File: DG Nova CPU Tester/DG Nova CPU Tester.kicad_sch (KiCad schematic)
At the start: 122 parts, among them J1 Slot_02x50_Odd_Even, J10 Programmed I/O, J11 CPU Option Inputs, J12 Data Channel, J13 Program Interrupt, J14 System Control, J17 CPU Option Outputs, J18 MEM Control Outputs, J19 Logic 8 CH, J20 Logic 8 CH, J21 Arduino Anolog Pins, J22 Arduino Digital Pins, J23 Arduino Digital Pins, J4 ATX Power Port, J6 MBO, J7 MEM, J8 Data Channel, J9 Front Panel Controls, SW1 Arduino Mega Reset, SW1 Pico Reset, SW2 Power Swtich, U1 74HC14, U2 Pico

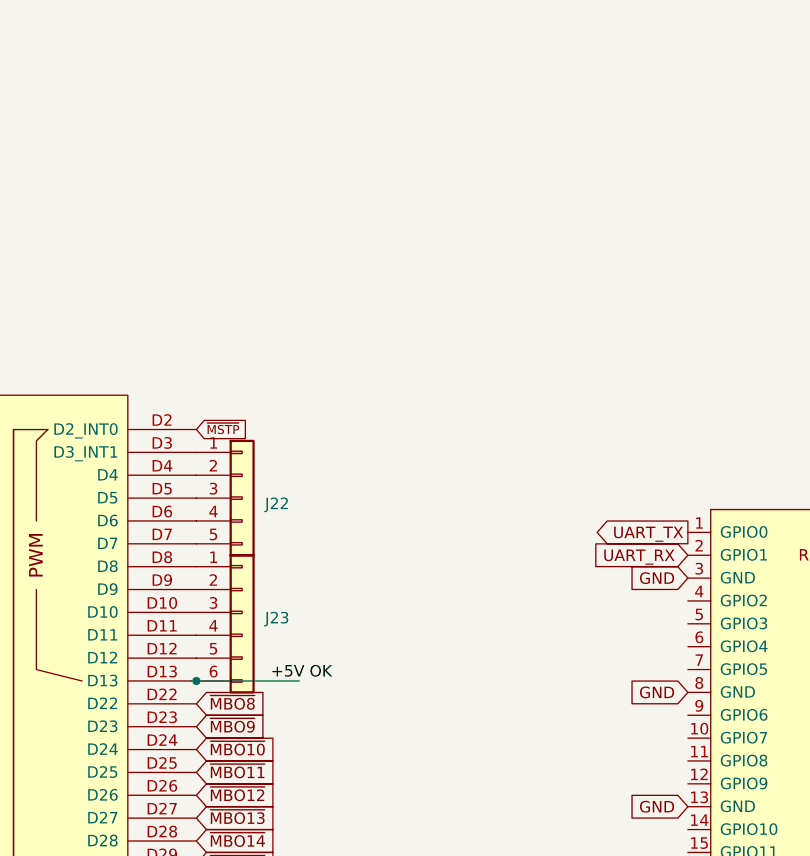
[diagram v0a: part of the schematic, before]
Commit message: repairs
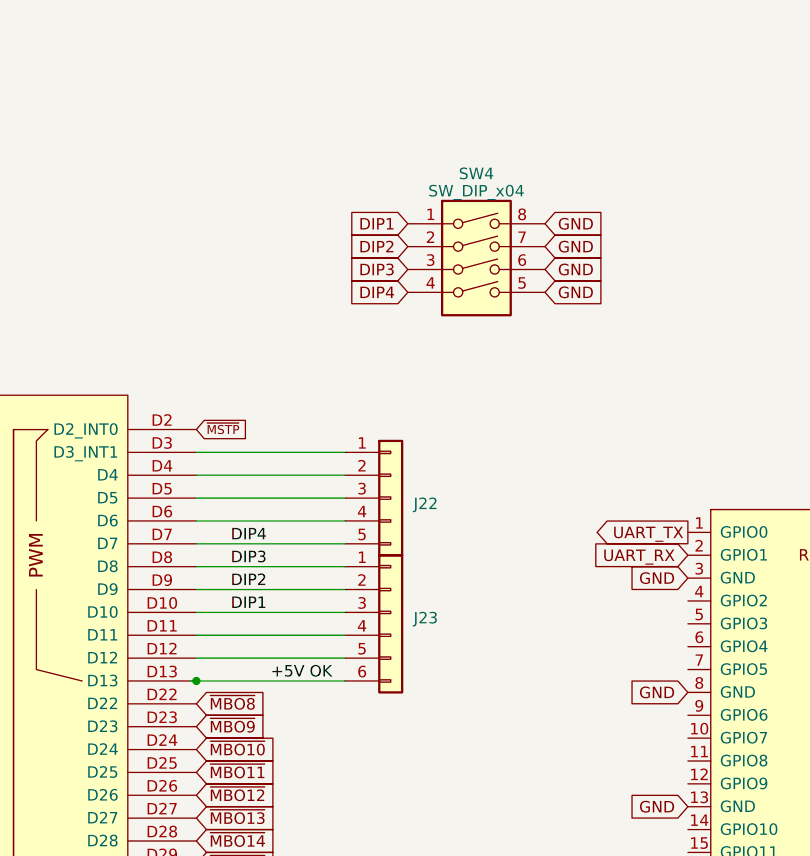
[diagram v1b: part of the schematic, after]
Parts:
- added SW4: SW_DIP_x04, Package_DIP:DIP-8_W7.62mm, symbol Switch:SW_DIP_x04
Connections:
- net GND: now also SW4.5, SW4.6, SW4.7, SW4.8
- net DIP1: now reaches J23.3 (Pin_3), XA1.D10
- net DIP1: now also SW4.1
- net DIP4: now reaches J22.5 (Pin_5), XA1.D7
- net DIP4: now also SW4.4
- net DIP3: now reaches J23.1 (Pin_1), XA1.D8
- net DIP3: now also SW4.3
- net DIP2: now reaches J23.2 (Pin_2), XA1.D9
- net DIP2: now also SW4.2
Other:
- moved on the sheet: J22, J23
